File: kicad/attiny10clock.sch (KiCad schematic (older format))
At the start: 41 parts, among them J1 USB_B_Micro, J2 Conn_02x04_Odd_Even, SW1 SW_DIP_x01, SW2 SW_DIP_x01, SW3 SW_DIP_x01, SW4 SW_DIP_x01, SW5 SW_DIP_x01, U1 ATtiny10-TS, U2 NPIC6C595, U3 NPIC6C595, U4 NPIC6C595, U5 NPIC6C595, U6 RT8097AHGB, X1 DFA-S15

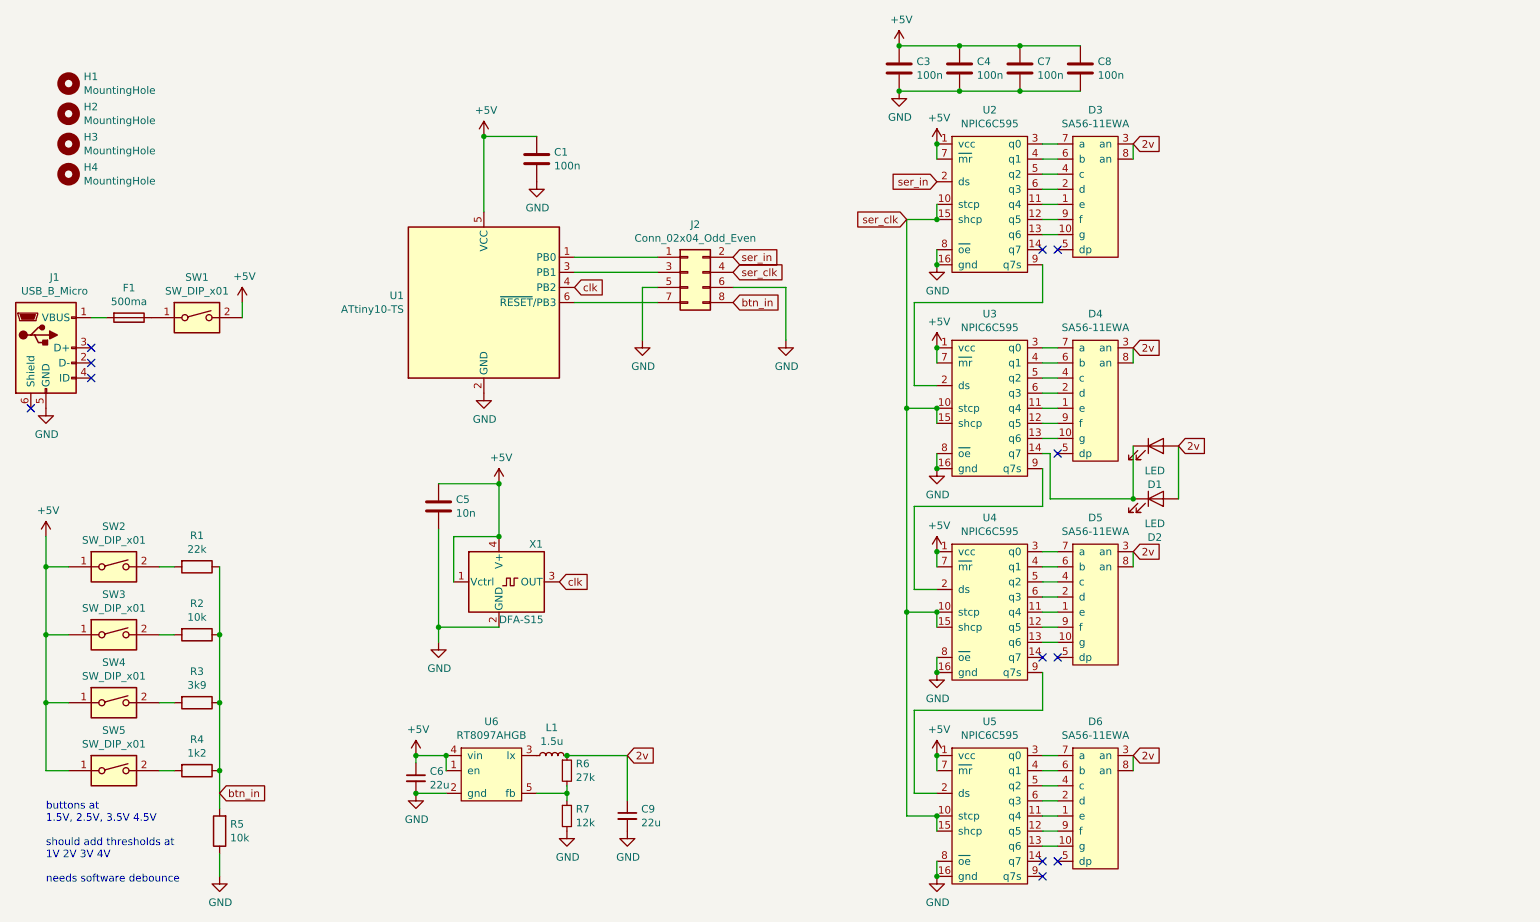
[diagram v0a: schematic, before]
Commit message: Finalize rev 2 pcb
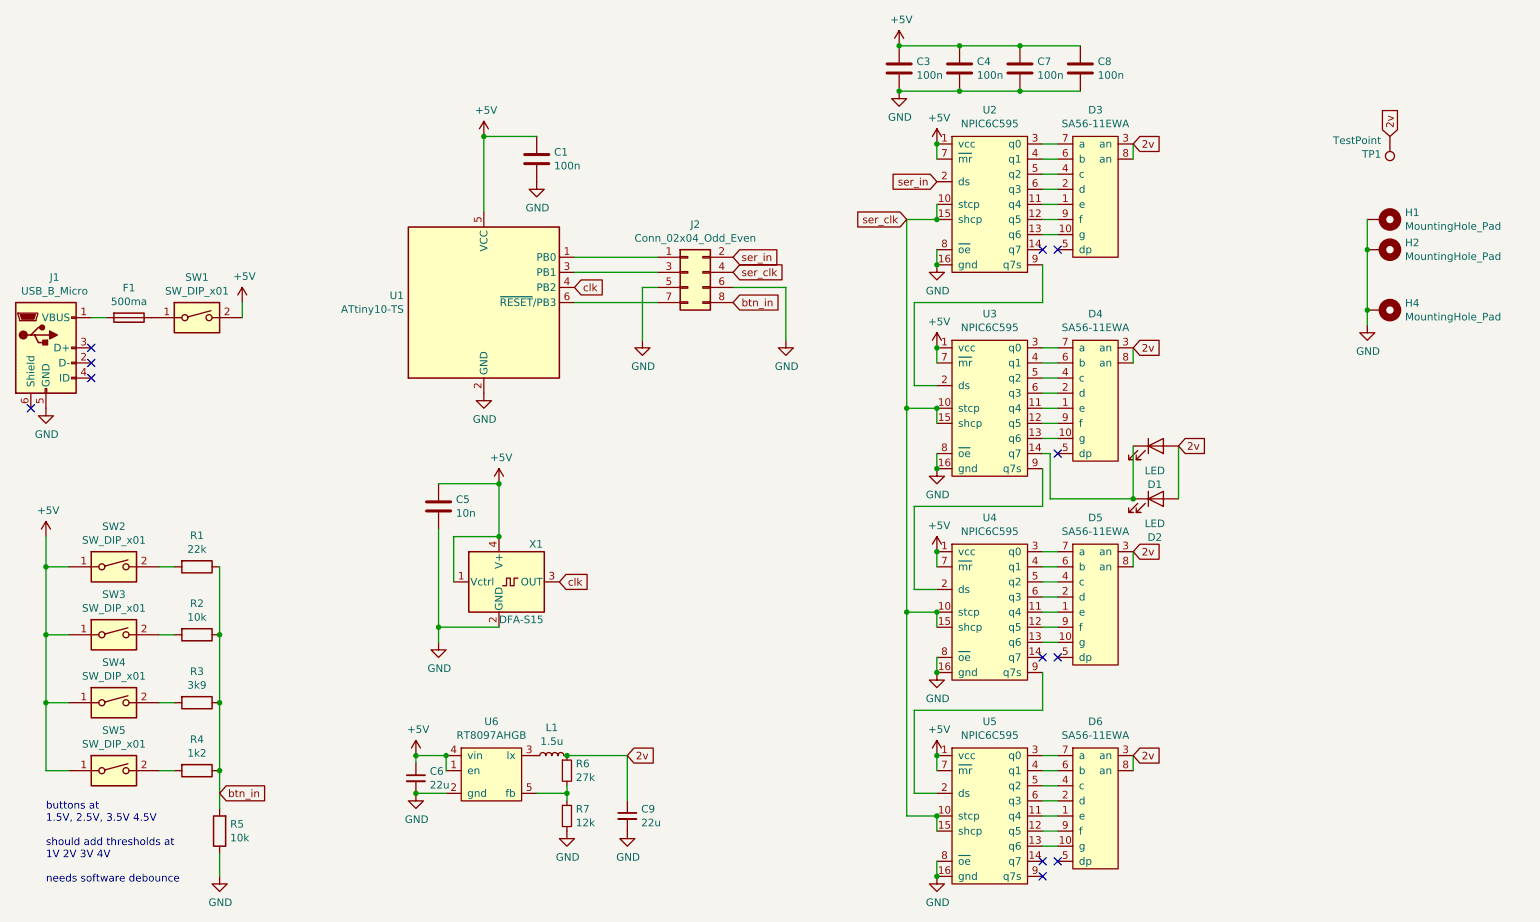
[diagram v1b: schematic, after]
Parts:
- removed H1, H2, H3, H4: MountingHole, MountingHole:MountingHole_2.2mm_M2, symbol Mechanical:MountingHole
- added H1, H2, H4: MountingHole_Pad, MountingHole:MountingHole_2.2mm_M2_Pad, symbol Mechanical:MountingHole_Pad
- added TP1: TestPoint, TestPoint:TestPoint_Pad_D2.0mm, symbol Connector:TestPoint
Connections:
- net 2v: now also TP1.1
- net GND: now also H1.1, H2.1, H4.1
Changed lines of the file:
@@
 	1    0    0    -1
 $EndComp
-Wire Wire Line
-	4650 5450 5050 5450
 Connection ~ 4650 5450
 Text GLabel 4700 2350 2    50   Input ~ 0
@@
 NoConn ~ 1100 3150
 $Comp
-L Mechanical:MountingHole H1
-U 1 1 6052C894
-P 1350 1000
-F 0 "H1" H 1450 1046 50  0000 L CNN
-F 1 "MountingHole" H 1450 955 50  0000 L CNN
-F 2 "MountingHole:MountingHole_2.2mm_M2" H 1350 1000 50  0001 C CNN
-F 3 "~" H 1350 1000 50  0001 C CNN
-	1    1350 1000
-	1    0    0    -1
-$EndComp
-$Comp
-L Mechanical:MountingHole H2
-U 1 1 6052D0D2
-P 1350 1200
-F 0 "H2" H 1450 1246 50  0000 L CNN
-F 1 "MountingHole" H 1450 1155 50  0000 L CNN
-F 2 "MountingHole:MountingHole_2.2mm_M2" H 1350 1200 50  0001 C CNN
-F 3 "~" H 1350 1200 50  0001 C CNN
-	1    1350 1200
-	1    0    0    -1
-$EndComp
-$Comp
-L Mechanical:MountingHole H3
-U 1 1 6052D545
-P 1350 1400
-F 0 "H3" H 1450 1446 50  0000 L CNN
-F 1 "MountingHole" H 1450 1355 50  0000 L CNN
-F 2 "MountingHole:MountingHole_2.2mm_M2" H 1350 1400 50  0001 C CNN
-F 3 "~" H 1350 1400 50  0001 C CNN
-	1    1350 1400
-	1    0    0    -1
-$EndComp
-$Comp
-L Mechanical:MountingHole H4
-U 1 1 6052D6A0
-P 1350 1600
-F 0 "H4" H 1450 1646 50  0000 L CNN
-F 1 "MountingHole" H 1450 1555 50  0000 L CNN
-F 2 "MountingHole:MountingHole_2.2mm_M2" H 1350 1600 50  0001 C CNN
-F 3 "~" H 1350 1600 50  0001 C CNN
-	1    1350 1600
-	1    0    0    -1
-$EndComp
+L Connector:TestPoint TP1
+U 1 1 6051D169
+P 10100 1350
+F 0 "TP1" H 10158 1468 50  0000 L CNN
+F 1 "TestPoint" H 10158 1377 50  0000 L CNN
+F 2 "TestPoint:TestPoint_Pad_D2.0mm" H 10300 1350 50  0001 C CNN
+F 3 "~" H 10300 1350 50  0001 C CNN
+	1    10100 1350
+	-1   0    0    1
+$EndComp
+Text GLabel 10100 1350 1    50   Input ~ 0
+2v
+Wire Wire Line
+	4650 5450 5050 5450
+$Comp
+L Mechanical:MountingHole_Pad H1
+U 1 1 60530F90
+P 10050 1900
+F 0 "H1" V 10004 2050 50  0000 L CNN
+F 1 "MountingHole_Pad" V 10095 2050 50  0000 L CNN
+F 2 "MountingHole:MountingHole_2.2mm_M2_Pad" H 10050 1900 50  0001 C CNN
+F 3 "~" H 10050 1900 50  0001 C CNN
+	1    10050 1900
+	0    1    1    0
+$EndComp
+$Comp
+L Mechanical:MountingHole_Pad H2
+U 1 1 60531C39
+P 10050 2100
+F 0 "H2" V 10004 2250 50  0000 L CNN
+F 1 "MountingHole_Pad" V 10095 2250 50  0000 L CNN
+F 2 "MountingHole:MountingHole_2.2mm_M2_Pad" H 10050 2100 50  0001 C CNN
+F 3 "~" H 10050 2100 50  0001 C CNN
+	1    10050 2100
+	0    1    1    0
+$EndComp
+$Comp
+L Mechanical:MountingHole_Pad H4
+U 1 1 60531F46
+P 10050 2500
+F 0 "H4" V 10004 2650 50  0000 L CNN
+F 1 "MountingHole_Pad" V 10095 2650 50  0000 L CNN
+F 2 "MountingHole:MountingHole_2.2mm_M2_Pad" H 10050 2500 50  0001 C CNN
+F 3 "~" H 10050 2500 50  0001 C CNN
+	1    10050 2500
+	0    1    1    0
+$EndComp
+Wire Wire Line
+	9950 1900 9950 2100
+Connection ~ 9950 2100
+$Comp
+L power:GND #PWR0103
+U 1 1 605410CB
+P 9950 2600
+F 0 "#PWR0103" H 9950 2350 50  0001 C CNN
+F 1 "GND" H 9955 2427 50  0000 C CNN
+F 2 "" H 9950 2600 50  0001 C CNN
+F 3 "" H 9950 2600 50  0001 C CNN
+	1    9950 2600
+	1    0    0    -1
+$EndComp
+Wire Wire Line
+	9950 2600 9950 2500
+Connection ~ 9950 2500
+Wire Wire Line
+	9950 2100 9950 2500
 $EndSCHEMATC

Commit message: Yey hardware works
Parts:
- D3, D4, D5, D6: symbol random_things:SA56-11EWA -> attiny10clock-rescue:SA56-11EWA-random_things
- U2, U3, U4, U5: symbol random_things:NPIC6C595 -> attiny10clock-rescue:NPIC6C595-random_things
- U6: symbol random_things:RT8097AHGB -> attiny10clock-rescue:RT8097AHGB-random_things
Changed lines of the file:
@@
 	8400 1400 8400 1500
 $Comp
-L random_things:SA56-11EWA D6
+L attiny10clock-rescue:SA56-11EWA-random_things D6
 U 1 1 604BC073
 P 8150 5800
@@
 NoConn ~ 7800 6150
 $Comp
-L random_things:NPIC6C595 U5
+L attiny10clock-rescue:NPIC6C595-random_things U5
 U 1 1 604BC068
 P 7450 5900
@@
 	7800 5450 7900 5450
 $Comp
-L random_things:SA56-11EWA D5
+L attiny10clock-rescue:SA56-11EWA-random_things D5
 U 1 1 604B56B5
 P 8150 4450
@@
 NoConn ~ 7800 4800
 $Comp
-L random_things:NPIC6C595 U4
+L attiny10clock-rescue:NPIC6C595-random_things U4
 U 1 1 604B56AA
 P 7450 4550
@@
 	7800 4100 7900 4100
 $Comp
-L random_things:SA56-11EWA D4
+L attiny10clock-rescue:SA56-11EWA-random_things D4
 U 1 1 604B2662
 P 8150 3100
@@
 NoConn ~ 7900 3450
 $Comp
-L random_things:NPIC6C595 U3
+L attiny10clock-rescue:NPIC6C595-random_things U3
 U 1 1 604B2657
 P 7450 3200
@@
 	7800 2750 7900 2750
 $Comp
-L random_things:SA56-11EWA D3
+L attiny10clock-rescue:SA56-11EWA-random_things D3
 U 1 1 6036F5A5
 P 8150 1750
@@
 NoConn ~ 7800 2100
 $Comp
-L random_things:NPIC6C595 U2
+L attiny10clock-rescue:NPIC6C595-random_things U2
 U 1 1 60492F39
 P 7450 1850
@@
 $EndComp
 $Comp
-L random_things:RT8097AHGB U6
+L attiny10clock-rescue:RT8097AHGB-random_things U6
 U 1 1 6059CE26
 P 4150 5550
